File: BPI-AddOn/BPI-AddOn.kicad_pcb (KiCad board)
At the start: 2 copper layers, 100 x 100 mm, 81 parts, among them CON1 BARREL_JACK, J1 RJ45, J2 RJ45, J3 RJ45, P1 DIN10-1, P10 CONN_01X03, P11 CONN_01X05, P12 CONN_01X05, P13 CONN_01X08, P15 CONN_02X11, P16 USB_B, P17 CONN_01X05, P18 CONN_01X05, P19 V, P2 DIN10-2, P20 - +, P21 USB_OTG, P22 CONN_01X06, P23 CONN_01X06, P24 CONN_02X02, P25 CONN_01X02, P3 DIN10-3, P4 DIN10-4, P5 DIN10-5, P6 DIN7-1, P7 DIN7-2, P8 DIN7-3, P9 CONN_01X03, U1 MC34063, U2 FT230XS

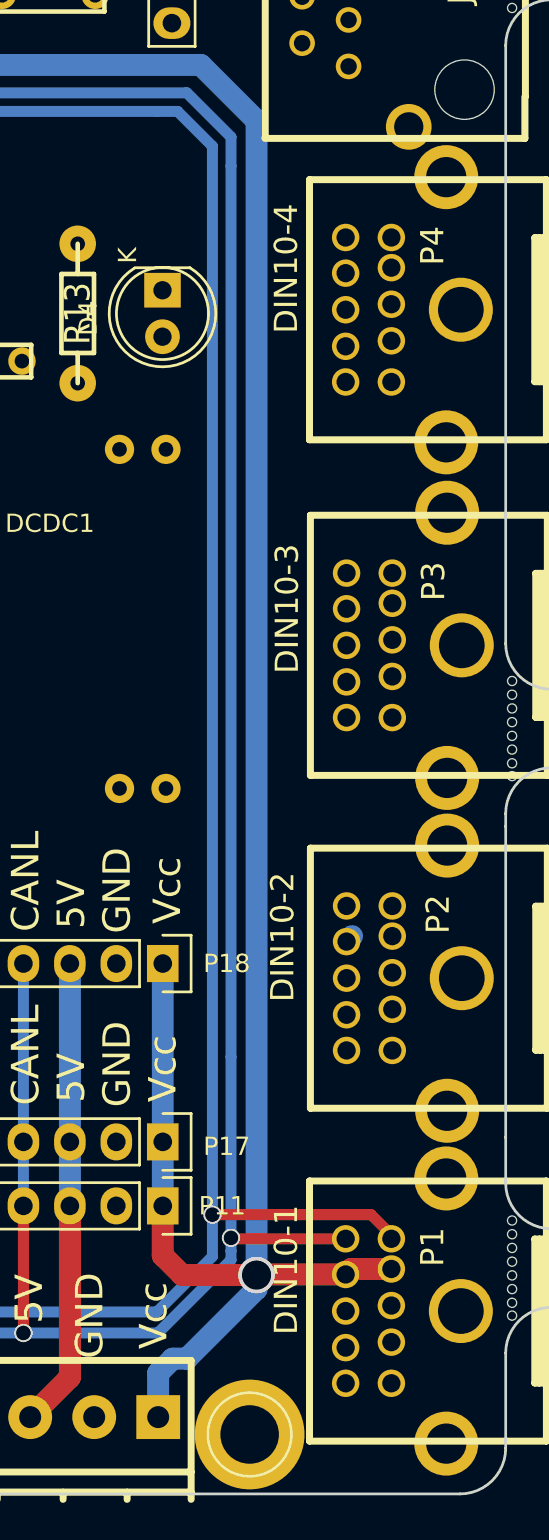
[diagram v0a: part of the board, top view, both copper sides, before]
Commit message: wip
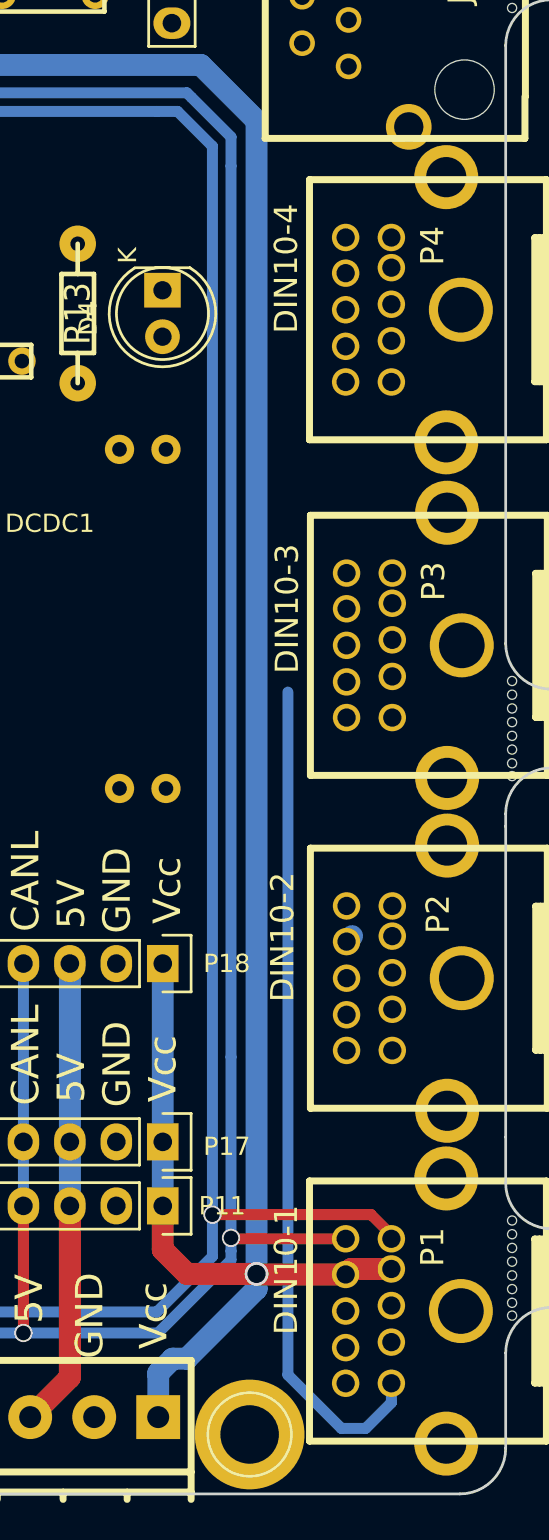
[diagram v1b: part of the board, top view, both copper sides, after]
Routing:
- net /GS0: track 0.00 -> 45.8 mm
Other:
- net class Vcc: via_dia 2 -> 1.3; via_drill 1.6 -> 1
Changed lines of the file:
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@@
-(kicad_pcb (version 4) (host pcbnew 4.0.2+e4-6225~38~ubuntu14.04.1-stable)
+(kicad_pcb (version 4) (host pcbnew 4.0.1-stable)
   (general
     (links 233)
     (no_connects 208)
-    (area 51.400001 38.02446 212.661501 154.700001)
+    (area 66.924999 48.924999 167.075001 149.075001)
     (thickness 1.6)
     (drawings 80)
-    (tracks 100)
+    (tracks 108)
     (zones 0)
     (modules 81)
@@
     (clearance 0.2)
     (trace_width 1.2)
-    (via_dia 2)
-    (via_drill 1.6)
-    (uvia_dia 1.3)
-    (uvia_drill 0.9)
+    (via_dia 1.3)
+    (via_drill 1)
+    (uvia_dia 0.6)
+    (uvia_drill 0.4)
     (add_net /5V)
     (add_net /J1_V)
@@
   (gr_line (start 69.5 149) (end 114.5 149) (angle 90) (layer Edge.Cuts) (width 0.15))
   (gr_line (start 69.5 49) (end 114.5 49) (angle 90) (layer Edge.Cuts) (width 0.15))
+  (segment (start 105.0925 142.494) (end 105.0925 105.156) (width 0.6) (layer B.Cu) (net 1))
+  (segment (start 108.0135 145.415) (end 105.0925 142.494) (width 0.6) (layer B.Cu) (net 1))
+  (segment (start 109.34566 145.415) (end 108.0135 145.415) (width 0.6) (layer B.Cu) (net 1))
+  (segment (start 110.75 142.95) (end 110.75 144.01066) (width 0.6) (layer B.Cu) (net 1))
+  (segment (start 110.75 144.01066) (end 109.34566 145.415) (width 0.6) (layer B.Cu) (net 1))
+  (segment (start 97.917 73.406) (end 84.201 73.406) (width 0.6) (layer B.Cu) (net 2))
   (segment (start 99.06 73.406) (end 97.917 73.406) (width 0.6) (layer B.Cu) (net 2))
-  (segment (start 97.917 73.406) (end 84.201 73.406) (width 0.6) (layer B.Cu) (net 2))
+  (segment (start 100.965 75.311) (end 99.06 73.406) (width 0.6) (layer B.Cu) (net 2))
+  (segment (start 84.201 73.406) (end 81.915 75.692) (width 0.6) (layer B.Cu) (net 2))
+  (segment (start 100.965 133.731) (end 100.965 75.311) (width 0.6) (layer B.Cu) (net 2))
   (segment (start 100.965 136.017) (end 100.965 133.731) (width 0.6) (layer B.Cu) (net 2))
-  (segment (start 100.965 133.731) (end 100.965 75.311) (width 0.6) (layer B.Cu) (net 2))
   (via (at 100.965 133.731) (size 1) (drill 0.8) (layers F.Cu B.Cu) (net 2))
   (segment (start 110.75 135.05) (end 110.75 134.84) (width 0.6) (layer F.Cu) (net 2))
@@
   (segment (start 109.64 133.73) (end 100.966 133.73) (width 0.6) (layer F.Cu) (net 2))
   (segment (start 100.966 133.73) (end 100.965 133.731) (width 0.6) (layer F.Cu) (net 2))
-  (segment (start 84.201 73.406) (end 81.915 75.692) (width 0.6) (layer B.Cu) (net 2))
-  (segment (start 100.965 75.311) (end 99.06 73.406) (width 0.6) (layer B.Cu) (net 2))
   (segment (start 97.932 139.05) (end 100.965 136.017) (width 0.6) (layer B.Cu) (net 2))
   (segment (start 87.99 139.05) (end 97.932 139.05) (width 0.6) (layer B.Cu) (net 2))
@@
   (segment (start 88.09 129.75) (end 88.09 120) (width 0.6) (layer B.Cu) (net 2))
   (segment (start 88.09 133.25) (end 88.09 129.75) (width 0.6) (layer B.Cu) (net 2))
+  (segment (start 83.947 72.39) (end 80.645 75.692) (width 0.6) (layer B.Cu) (net 3))
+  (segment (start 99.568 72.39) (end 83.947 72.39) (width 0.6) (layer B.Cu) (net 3))
+  (segment (start 99.822 72.644) (end 99.568 72.39) (width 0.6) (layer B.Cu) (net 3))
   (segment (start 101.981 74.803) (end 99.822 72.644) (width 0.6) (layer B.Cu) (net 3))
-  (segment (start 99.822 72.644) (end 99.568 72.39) (width 0.6) (layer B.Cu) (net 3))
+  (segment (start 101.981 125.095) (end 101.981 76.409612) (width 0.6) (layer B.Cu) (net 3))
+  (segment (start 101.981 135.001) (end 101.981 125.095) (width 0.6) (layer B.Cu) (net 3))
+  (segment (start 101.981 76.409612) (end 101.981 74.803) (width 0.6) (layer B.Cu) (net 3))
   (segment (start 101.981 135.708106) (end 101.981 135.001) (width 0.6) (layer B.Cu) (net 3))
   (segment (start 101.981 136.209998) (end 101.981 135.708106) (width 0.6) (layer B.Cu) (net 3))
   (segment (start 90.63 140.2) (end 97.990998 140.2) (width 0.6) (layer B.Cu) (net 3))
   (segment (start 97.990998 140.2) (end 101.981 136.209998) (width 0.6) (layer B.Cu) (net 3))
-  (segment (start 101.981 135.001) (end 101.981 125.095) (width 0.6) (layer B.Cu) (net 3))
   (via (at 101.981 135.001) (size 1) (drill 0.8) (layers F.Cu B.Cu) (net 3))
   (segment (start 108.25 135.05) (end 102.03 135.05) (width 0.6) (layer F.Cu) (net 3))
   (segment (start 102.03 135.05) (end 101.981 135.001) (width 0.6) (layer F.Cu) (net 3))
-  (segment (start 83.947 72.39) (end 80.645 75.692) (width 0.6) (layer B.Cu) (net 3))
-  (segment (start 99.568 72.39) (end 83.947 72.39) (width 0.6) (layer B.Cu) (net 3))
-  (segment (start 101.981 76.409612) (end 101.981 74.803) (width 0.6) (layer B.Cu) (net 3))
-  (segment (start 101.981 125.095) (end 101.981 76.409612) (width 0.6) (layer B.Cu) (net 3))
   (segment (start 90.63 133.25) (end 90.63 140.2) (width 0.6) (layer F.Cu) (net 3))
   (via (at 90.63 140.2) (size 1) (drill 0.8) (layers F.Cu B.Cu) (net 3))
@@
   (segment (start 152.78 134.72) (end 152.78 126.5) (width 0.6) (layer B.Cu) (net 20))
   (segment (start 150.38 137.12) (end 152.78 134.72) (width 0.6) (layer B.Cu) (net 20))
-  (segment (start 99.314 137.033) (end 98.25 135.969) (width 1.2) (layer F.Cu) (net 22))
-  (segment (start 98.25 135.969) (end 98.25 133.25) (width 1.2) (layer F.Cu) (net 22))
-  (segment (start 103.378 137.033) (end 99.314 137.033) (width 1.2) (layer F.Cu) (net 22))
-  (segment (start 103.411 137) (end 103.378 137.033) (width 1.2) (layer F.Cu) (net 22))
-  (segment (start 108.25 137) (end 103.411 137) (width 1.2) (layer F.Cu) (net 22))
-  (via (at 103.378 137.033) (size 2) (drill 1.6) (layers F.Cu B.Cu) (net 22))
   (segment (start 82.482999 71.695001) (end 79.248 74.93) (width 1.2) (layer B.Cu) (net 22))
+  (segment (start 103.378 73.914) (end 100.33 70.866) (width 1.2) (layer B.Cu) (net 22))
   (segment (start 83.312 70.866) (end 82.482999 71.695001) (width 1.2) (layer B.Cu) (net 22))
   (segment (start 100.33 70.866) (end 83.312 70.866) (width 1.2) (layer B.Cu) (net 22))
-  (segment (start 103.378 73.914) (end 100.33 70.866) (width 1.2) (layer B.Cu) (net 22))
-  (segment (start 103.378 137.795) (end 103.378 73.914) (width 1.2) (layer B.Cu) (net 22))
+  (segment (start 103.378 137.033) (end 103.378 73.914) (width 1.2) (layer B.Cu) (net 22))
+  (segment (start 103.378 136.9695) (end 99.568 136.9695) (width 1.2) (layer F.Cu) (net 22))
+  (segment (start 98.25 135.6515) (end 98.25 133.25) (width 1.2) (layer F.Cu) (net 22) (status 800000))
+  (segment (start 99.568 136.9695) (end 98.25 135.6515) (width 1.2) (layer F.Cu) (net 22))
+  (segment (start 108.25 137) (end 103.4085 137) (width 1.2) (layer F.Cu) (net 22) (status 400000))
+  (segment (start 103.4415 137.033) (end 103.378 137.033) (width 1.2) (layer B.Cu) (net 22))
+  (segment (start 103.378 136.9695) (end 103.4415 137.033) (width 1.2) (layer B.Cu) (net 22))
+  (via (at 103.378 136.9695) (size 1.3) (drill 1) (layers F.Cu B.Cu) (net 22))
+  (segment (start 103.4085 137) (end 103.378 136.9695) (width 1.2) (layer F.Cu) (net 22))
+  (segment (start 103.378 137.795) (end 103.378 137.033) (width 1.2) (layer B.Cu) (net 22))
   (segment (start 99.568 141.605) (end 103.378 137.795) (width 1.2) (layer B.Cu) (net 22))
   (segment (start 98.795 141.605) (end 99.568 141.605) (width 1.2) (layer B.Cu) (net 22))
+  (segment (start 98 144.8) (end 98 142.4) (width 1.2) (layer B.Cu) (net 22))
+  (segment (start 98 142.4) (end 98.795 141.605) (width 1.2) (layer B.Cu) (net 22))
   (segment (start 110.75 136.7) (end 108.55 136.7) (width 1.2) (layer F.Cu) (net 22))
   (segment (start 108.55 136.7) (end 108.25 137) (width 1.2) (layer F.Cu) (net 22))
@@
   (segment (start 98.25 133.25) (end 98.25 129.75) (width 1.2) (layer B.Cu) (net 22))
   (segment (start 108.6 118.5) (end 108.3 118.8) (width 1.2) (layer B.Cu) (net 22))
-  (segment (start 98 144.8) (end 98 142.4) (width 1.2) (layer B.Cu) (net 22))
-  (segment (start 98 142.4) (end 98.795 141.605) (width 1.2) (layer B.Cu) (net 22))
   (segment (start 98.9024 68.58) (end 98.75 68.58) (width 1.2) (layer B.Cu) (net 22))
   (segment (start 98 133.5) (end 98.25 133.25) (width 0.6) (layer B.Cu) (net 22))
